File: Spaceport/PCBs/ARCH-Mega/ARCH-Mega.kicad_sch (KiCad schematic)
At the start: 93 parts, among them J1 Conn_01x04_Pin, J2 Conn_01x05_Pin, J3 Charge, J4 USB_C_Receptacle_USB2.0_16P, J5 BAT, J6 SW, Q1 PMOS, U1 STM32C011F6U6TR, U2 TPS61288LRQQR, U3 TPS51388VABR, U4 LDL212PVR, U6 BQ25308RTER

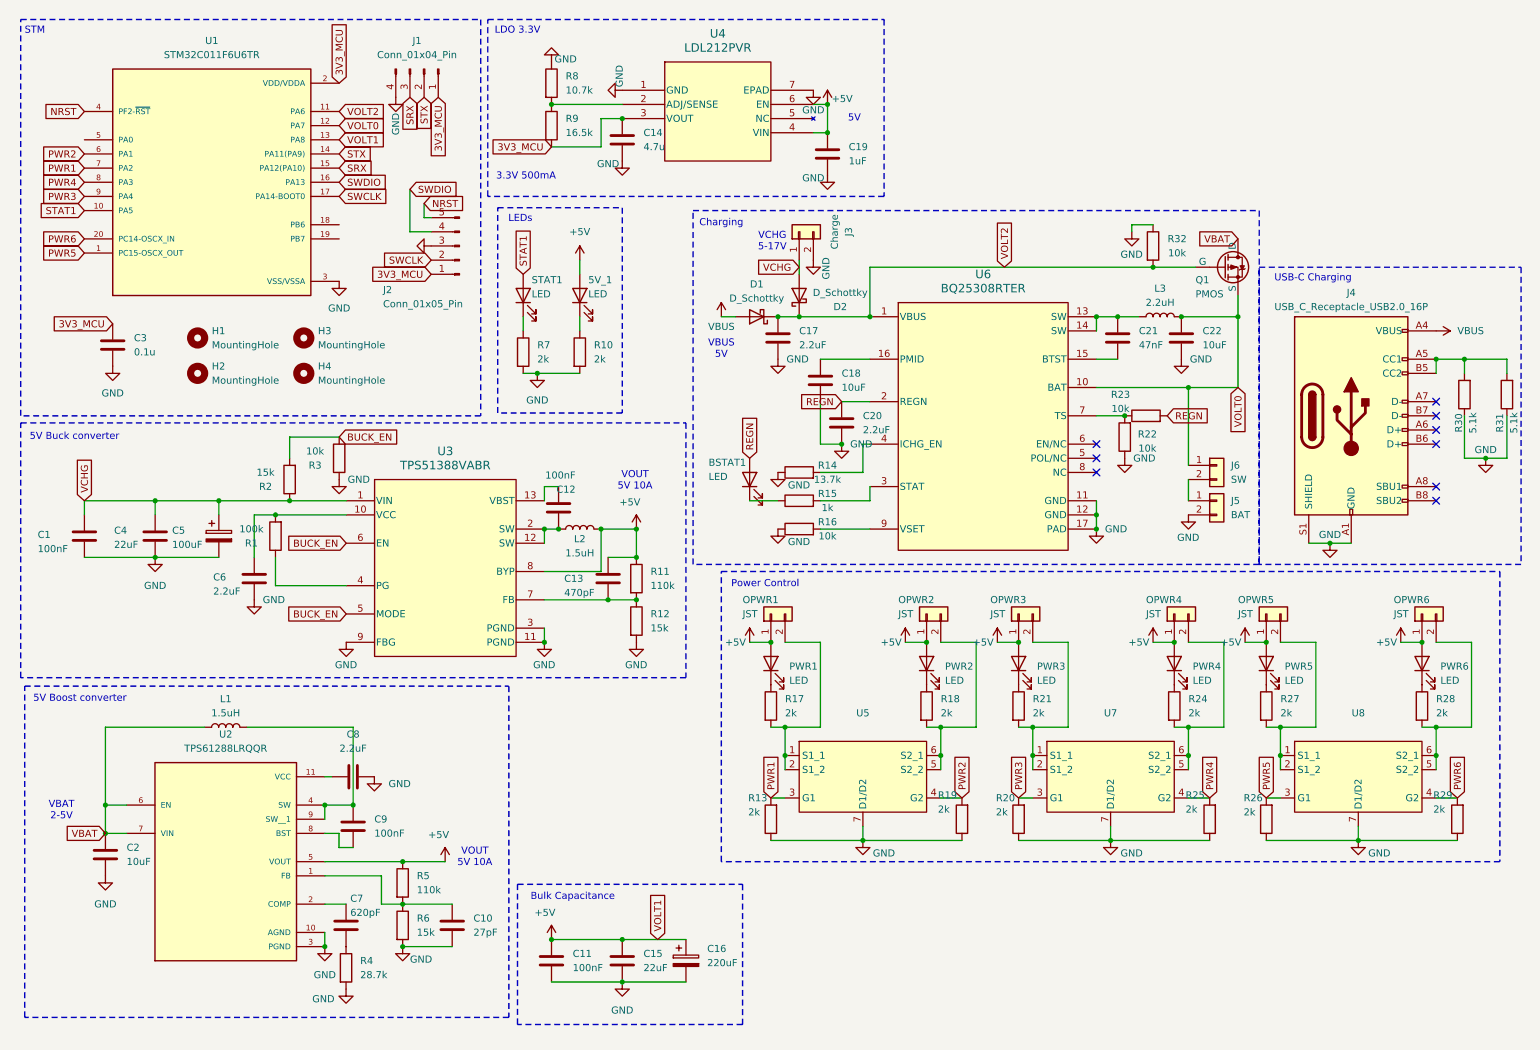
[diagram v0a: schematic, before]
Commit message: ARCH-Mega pre USB PD
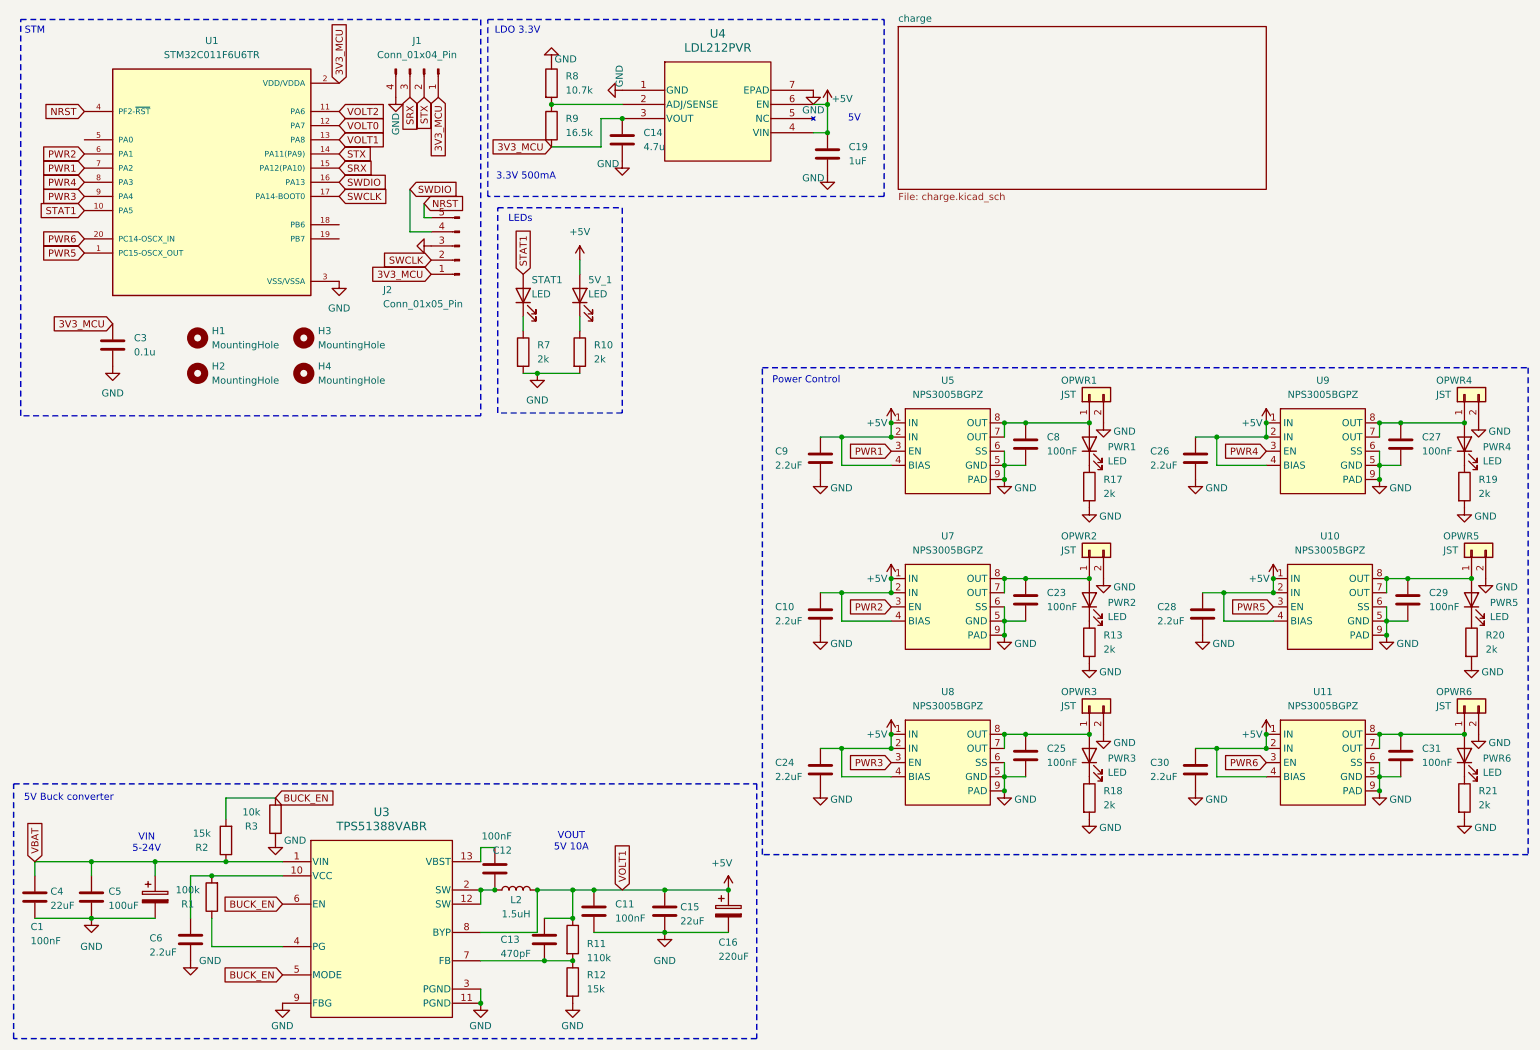
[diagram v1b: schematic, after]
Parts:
- removed BSTAT1: LED, LED_SMD:LED_0805_2012Metric_Pad1.15x1.40mm_HandSolder, symbol Device:LED
- removed C17, C20: 2.2uF, Capacitor_SMD:C_0805_2012Metric, symbol Device:C
- removed C18, C2, C22: 10uF, Capacitor_SMD:C_0603_1608Metric, symbol Device:C
- removed C21: 47nF, Capacitor_SMD:C_0805_2012Metric, symbol Device:C
- removed C7: 620pF, Capacitor_SMD:C_0603_1608Metric, symbol Device:C
- removed D1, D2: D_Schottky, Avionics:Schottky_3A_DO-214AC_SMA, symbol Device:D_Schottky
- removed J3: Charge, Avionics:JST_XH_1x2_P2.50mm_Horizontal_Small, symbol Connector_Generic:Conn_01x02
- removed J4: USB_C_Receptacle_USB2.0_16P, Connector_USB:USB_C_Receptacle_GCT_USB4105-xx-A_16P_TopMnt_Horizontal, symbol Connector:USB_C_Receptacle_USB2.0_16P
- removed J5: BAT, Avionics:JST_XH_1x2_P2.50mm_Horizontal_Small, symbol Connector_Generic:Conn_01x02
- removed J6: SW, Avionics:JST_XH_1x2_P2.50mm_Horizontal_Small, symbol Connector_Generic:Conn_01x02
- removed L1: 1.5uH, Avionics:HCM1A1305, symbol Device:L
- removed L3: 2.2uH, Avionics:IND_AMRM00101040_PUL, symbol Device:L
- removed Q1: PMOS, Avionics:SI7615ADN-T1-GE3, symbol Simulation_SPICE:PMOS
- removed R14: 13.7k, Resistor_SMD:R_0603_1608Metric, symbol Device:R
- removed R15: 1k, Resistor_SMD:R_0603_1608Metric, symbol Device:R
- removed R16, R22, R23, R32: 10k, Resistor_SMD:R_0603_1608Metric, symbol Device:R
- removed R24, R25, R26, R27, R28, R29: 2k, Resistor_SMD:R_0603_1608Metric, symbol Device:R
- removed R30, R31: 5.1k, Resistor_SMD:R_0402_1005Metric, symbol Device:R
- removed R4: 28.7k, Resistor_SMD:R_0603_1608Metric, symbol Device:R
- removed R5: 110k, Resistor_SMD:R_0603_1608Metric, symbol Device:R
- removed R6: 15k, Resistor_SMD:R_0603_1608Metric, symbol Device:R
- removed U2: TPS61288LRQQR, Avionics:CONV_TPS61288LRQQR, symbol SRAD-Avionics:TPS61288LRQQR
- removed U5, U7, U8: ~, Package_DFN_QFN:DFN-6-1EP_3x2mm_P0.5mm_EP1.65x1.35mm, symbol Avionics:GSFN0232
- removed U6: BQ25308RTER, Avionics:BQ25308RTER, symbol Avionics:BQ25308RTER
- added C23, C25, C27, C29, C31: 100nF, Capacitor_SMD:C_0603_1608Metric, symbol Device:C
- added C24, C26, C28, C30: 2.2uF, Capacitor_SMD:C_0603_1608Metric, symbol Device:C
- added U10, U11, U5, U7, U8, U9: NPS3005BGPZ, Package_SON:Texas_DSG0008A_WSON-8-1EP_2x2mm_P0.5mm_EP0.9x1.6mm, symbol Avionics:NPS3005BGPZ
- C10: value 27pF -> 2.2uF
- C8: value 2.2uF -> 100nF; footprint Capacitor_SMD:C_0805_2012Metric -> Capacitor_SMD:C_0603_1608Metric
- C9: value 100nF -> 2.2uF
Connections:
- net VCHG is gone; now on net VBAT: C1.1, C4.1, C5.1, R2.1, U3.1 (VIN)
- net +5V: now also C10.2, C9.2, C24.2, C26.2, C28.2, C30.2, U10.1 (IN), U10.2 (IN), U10.4 (BIAS), U11.1 (IN), U11.2 (IN), U11.4 (BIAS), U5.1 (IN), U5.2 (IN), U5.4 (BIAS), U7.1 (IN), U7.2 (IN), U7.4 (BIAS), U8.1 (IN), U8.2 (IN), U8.4 (BIAS), U9.1 (IN), U9.2 (IN), U9.4 (BIAS); no longer OPWR1.1 (Pin_1), OPWR2.1 (Pin_1), OPWR3.1 (Pin_1), OPWR4.1 (Pin_1), OPWR5.1 (Pin_1), OPWR6.1 (Pin_1), PWR1.2 (A), PWR2.2 (A), PWR3.2 (A), PWR4.2 (A), PWR5.2 (A), PWR6.2 (A)
- net GND: now also C10.1, C8.1, C9.1, OPWR1.2 (Pin_2), OPWR2.2 (Pin_2), OPWR3.2 (Pin_2), OPWR4.2 (Pin_2), OPWR5.2 (Pin_2), OPWR6.2 (Pin_2), R13.2, R17.2, R18.2, R19.2, R20.2, R21.2, C23.1, C24.1, C25.1, C26.1, C27.1, C28.1, C29.1, C30.1, C31.1, U10.5 (GND), U10.6 (SS), U10.9 (PAD), U11.5 (GND), U11.6 (SS), U11.9 (PAD), U5.5 (GND), U5.6 (SS), U5.9 (PAD), U7.5 (GND), U7.6 (SS), U7.9 (PAD), U8.5 (GND), U8.6 (SS), U8.9 (PAD), U9.5 (GND), U9.6 (SS), U9.9 (PAD); no longer C10.2, C8.2, R13.1, R19.1, R20.1
- net PWR1: now also U5.3 (EN); no longer R13.2
- net PWR2: now also U7.3 (EN); no longer R19.2
- net PWR3: now also U8.3 (EN); no longer R20.2
- net PWR4: now also U9.3 (EN)
- net PWR5: now also U10.3 (EN)
- net PWR6: now also U11.3 (EN)
- net at PWR5.1 (K): now also R20.1
- net at PWR6.1 (K): now also R21.1
- net at R18.1: now also PWR3.1 (K); no longer PWR2.1 (K)
- net at PWR4.1 (K): now also R19.1
- new net: C25.2, OPWR3.1 (Pin_1), PWR3.2 (A), U8.7 (OUT), U8.8 (OUT)
- new net: C8.2, OPWR1.1 (Pin_1), PWR1.2 (A), U5.7 (OUT), U5.8 (OUT)
- new net: C29.2, OPWR5.1 (Pin_1), PWR5.2 (A), U10.7 (OUT), U10.8 (OUT)
- new net: C23.2, OPWR2.1 (Pin_1), PWR2.2 (A), U7.7 (OUT), U7.8 (OUT)
- new net: C31.2, OPWR6.1 (Pin_1), PWR6.2 (A), U11.7 (OUT), U11.8 (OUT)
- new net: C27.2, OPWR4.1 (Pin_1), PWR4.2 (A), U9.7 (OUT), U9.8 (OUT)
- new net: PWR2.1 (K), R13.1
- no-connect marks 9 -> 0
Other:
- added sheet charge (charge.kicad_sch)
- note added: "VIN 5-24V"
- note removed: "5V Boost converter"
- note removed: "Bulk Capacitance"
- note removed: "Charging"
- note removed: "USB-C Charging"
- note removed: "VBAT 2-5V"
- note removed: "VBUS 5V"
- note removed: "VCHG 5-17V"
- moved on the sheet: C1, C11, C12, C13, C15, C16, C4, C5, C6, L2, OPWR1, PWR1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
